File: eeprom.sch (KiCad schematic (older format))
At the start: 7 parts, among them U3 24LC01

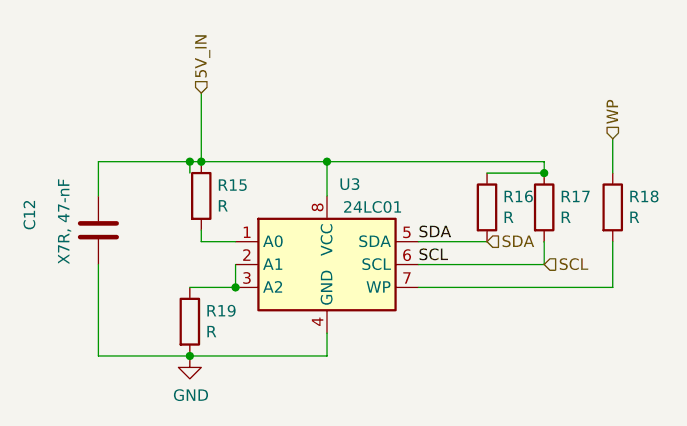
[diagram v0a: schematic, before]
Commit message: add voltage supply sense resistors
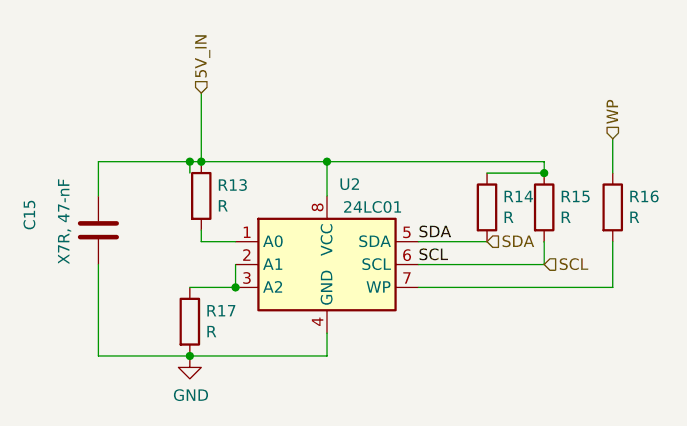
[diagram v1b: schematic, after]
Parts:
- renumbered C12 to C15, R15 to R13, R16 to R14, R17 to R15, R18 to R16, R19 to R17, U3 to U2
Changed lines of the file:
@@
 P 4310 3200
 AR Path="/60E74488/60F67DC6" Ref="U?"  Part="1"
-AR Path="/60F66E2D/60F67DC6" Ref="U3"  Part="1"
-F 0 "U3" H 4410 3550 50  0000 C CNN
+AR Path="/60F66E2D/60F67DC6" Ref="U2"  Part="1"
+F 0 "U2" H 4410 3550 50  0000 C CNN
 F 1 "24LC01" H 4510 3450 50  0000 C CNN
 F 2 "Package_DFN_QFN:DFN-8-1EP_3x2mm_P0.5mm_EP1.36x1.46mm" H 4310 3200 50  0001 C CNN
@@
 P 3760 2900
 AR Path="/60E74488/60F67DCC" Ref="R?"  Part="1"
-AR Path="/60F66E2D/60F67DCC" Ref="R15"  Part="1"
-F 0 "R15" H 3830 2946 50  0000 L CNN
+AR Path="/60F66E2D/60F67DCC" Ref="R13"  Part="1"
+F 0 "R13" H 3830 2946 50  0000 L CNN
 F 1 "R" H 3830 2855 50  0000 L CNN
 F 2 "Resistor_SMD:R_0603_1608Metric_Pad1.05x0.95mm_HandSolder" V 3690 2900 50  0001 C CNN
@@
 P 3710 3450
 AR Path="/60E74488/60F67DD8" Ref="R?"  Part="1"
-AR Path="/60F66E2D/60F67DD8" Ref="R19"  Part="1"
-F 0 "R19" H 3780 3496 50  0000 L CNN
+AR Path="/60F66E2D/60F67DD8" Ref="R17"  Part="1"
+F 0 "R17" H 3780 3496 50  0000 L CNN
 F 1 "R" H 3780 3405 50  0000 L CNN
 F 2 "Resistor_SMD:R_0603_1608Metric_Pad1.05x0.95mm_HandSolder" V 3640 3450 50  0001 C CNN
@@
 P 3710 3600
 AR Path="/60E74488/60F67DDE" Ref="#PWR?"  Part="1"
-AR Path="/60F66E2D/60F67DDE" Ref="#PWR0102"  Part="1"
-F 0 "#PWR0102" H 3710 3350 50  0001 C CNN
+AR Path="/60F66E2D/60F67DDE" Ref="#PWR015"  Part="1"
+F 0 "#PWR015" H 3710 3350 50  0001 C CNN
 F 1 "GND" H 3715 3427 50  0000 C CNN
 F 2 "" H 3710 3600 50  0001 C CNN
@@
 P 5010 2950
 AR Path="/60E74488/60F67DE4" Ref="R?"  Part="1"
-AR Path="/60F66E2D/60F67DE4" Ref="R16"  Part="1"
-F 0 "R16" H 5080 2996 50  0000 L CNN
+AR Path="/60F66E2D/60F67DE4" Ref="R14"  Part="1"
+F 0 "R14" H 5080 2996 50  0000 L CNN
 F 1 "R" H 5080 2905 50  0000 L CNN
 F 2 "Resistor_SMD:R_0603_1608Metric_Pad1.05x0.95mm_HandSolder" V 4940 2950 50  0001 C CNN
@@
 P 5260 2950
 AR Path="/60E74488/60F67DEA" Ref="R?"  Part="1"
-AR Path="/60F66E2D/60F67DEA" Ref="R17"  Part="1"
-F 0 "R17" H 5330 2996 50  0000 L CNN
+AR Path="/60F66E2D/60F67DEA" Ref="R15"  Part="1"
+F 0 "R15" H 5330 2996 50  0000 L CNN
 F 1 "R" H 5330 2905 50  0000 L CNN
 F 2 "Resistor_SMD:R_0603_1608Metric_Pad1.05x0.95mm_HandSolder" V 5190 2950 50  0001 C CNN
@@
 P 3310 3050
 AR Path="/60E74488/60F67DF8" Ref="C?"  Part="1"
-AR Path="/60F66E2D/60F67DF8" Ref="C12"  Part="1"
-F 0 "C12" V 3010 3050 50  0000 L CNN
+AR Path="/60F66E2D/60F67DF8" Ref="C15"  Part="1"
+F 0 "C15" V 3010 3050 50  0000 L CNN
 F 1 "X7R, 47-nF" V 3160 2900 50  0000 L CNN
 F 2 "Capacitor_SMD:C_0603_1608Metric_Pad1.05x0.95mm_HandSolder" H 3348 2900 50  0001 C CNN
@@
 P 5560 2950
 AR Path="/60E74488/60F67E0E" Ref="R?"  Part="1"
-AR Path="/60F66E2D/60F67E0E" Ref="R18"  Part="1"
-F 0 "R18" H 5630 2996 50  0000 L CNN
+AR Path="/60F66E2D/60F67E0E" Ref="R16"  Part="1"
+F 0 "R16" H 5630 2996 50  0000 L CNN
 F 1 "R" H 5630 2905 50  0000 L CNN
 F 2 "Resistor_SMD:R_0603_1608Metric_Pad1.05x0.95mm_HandSolder" V 5490 2950 50  0001 C CNN
